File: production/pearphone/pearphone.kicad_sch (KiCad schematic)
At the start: 3 parts, among them SW1 SW_Push, U2 XIAO_ESP32C3

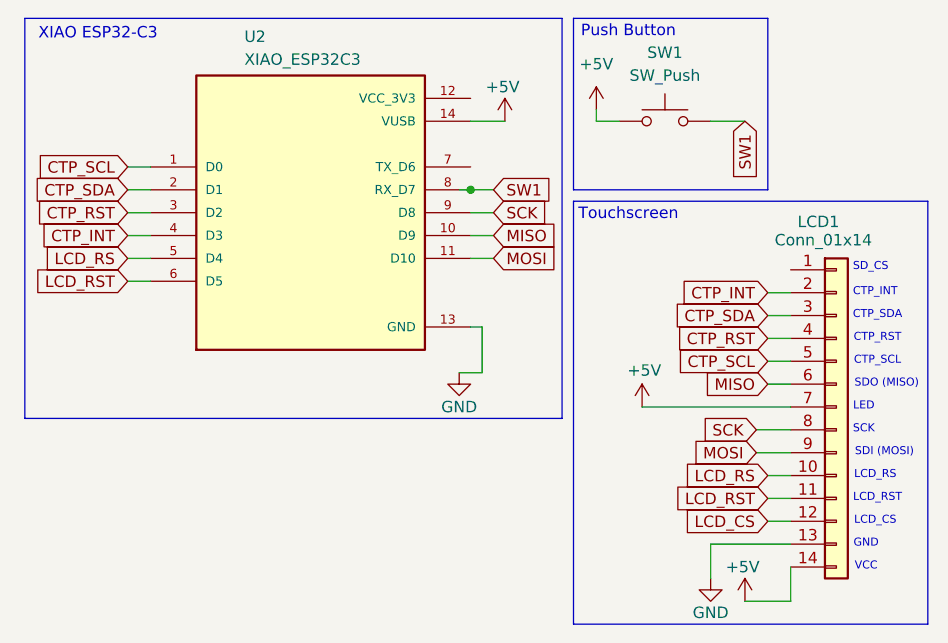
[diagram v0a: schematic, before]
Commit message: Revised schematic
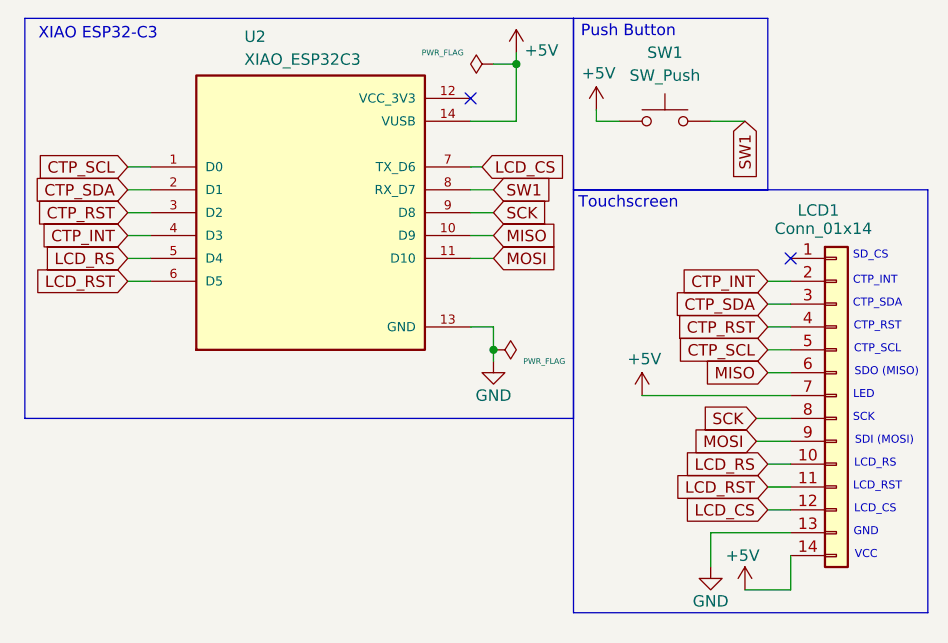
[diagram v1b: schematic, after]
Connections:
- net LCD_CS: now also U2.7 (TX_D6)
- no-connect marks 0 -> 2
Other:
- moved on the sheet: LCD1

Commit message: Placed components on PCB
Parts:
- LCD1: footprint (none) -> Connector_PinSocket_2.54mm:PinSocket_1x14_P2.54mm_Vertical
- SW1: footprint (none) -> Button_Switch_THT:SW_PUSH_6mm
- U2: footprint XIAO_ESP32C3:MODULE_XIAO_ESP32C3 -> footprints:MODULE_XIAO_ESP32C3
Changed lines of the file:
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@@
 			)
 		)
-		(property "Footprint" "XIAO_ESP32C3:MODULE_XIAO_ESP32C3"
+		(property "Footprint" "footprints:MODULE_XIAO_ESP32C3"
 			(at 44.45 34.29 0)
 			(hide yes)
@@
 			)
 		)
-		(property "Footprint" ""
+		(property "Footprint" "Button_Switch_THT:SW_PUSH_6mm"
 			(at 83.82 19.05 0)
 			(hide yes)
@@
 			)
 		)
-		(property "Footprint" ""
+		(property "Footprint" "Connector_PinSocket_2.54mm:PinSocket_1x14_P2.54mm_Vertical"
 			(at 102.87 54.61 0)
 			(hide yes)
